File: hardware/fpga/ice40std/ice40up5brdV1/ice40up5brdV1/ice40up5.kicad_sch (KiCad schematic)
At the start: 5 parts, among them U1 ICE40UP5K-SG48ITR

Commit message: pwm / lvds power / filters
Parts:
- C1, C20: footprint Capacitor_SMD:C_0402_1005Metric -> Capacitor_SMD:C_1206_3216Metric
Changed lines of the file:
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@@
       (effects (font (size 1.27 1.27)) (justify left))
     )
-    (property "Footprint" "Capacitor_SMD:C_0402_1005Metric" (id 2) (at 127.9652 53.34 0)
+    (property "Footprint" "Capacitor_SMD:C_1206_3216Metric" (id 2) (at 127.9652 53.34 0)
       (effects (font (size 1.27 1.27)) hide)
     )
@@
       (effects (font (size 1.27 1.27)) (justify left))
     )
-    (property "Footprint" "Capacitor_SMD:C_0402_1005Metric" (id 2) (at 238.4552 58.4075 0)
+    (property "Footprint" "Capacitor_SMD:C_1206_3216Metric" (id 2) (at 238.4552 58.4075 0)
       (effects (font (size 1.27 1.27)) hide)
     )

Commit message: pwm / lvds power / filters
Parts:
- C1, C20: footprint Capacitor_SMD:C_1206_3216Metric -> Capacitor_SMD:C_0603_1608Metric
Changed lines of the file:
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@@
       (effects (font (size 1.27 1.27)) (justify left))
     )
-    (property "Footprint" "Capacitor_SMD:C_1206_3216Metric" (id 2) (at 127.9652 53.34 0)
+    (property "Footprint" "Capacitor_SMD:C_0603_1608Metric" (id 2) (at 127.9652 53.34 0)
       (effects (font (size 1.27 1.27)) hide)
     )
@@
       (effects (font (size 1.27 1.27)) (justify left))
     )
-    (property "Footprint" "Capacitor_SMD:C_1206_3216Metric" (id 2) (at 238.4552 58.4075 0)
+    (property "Footprint" "Capacitor_SMD:C_0603_1608Metric" (id 2) (at 238.4552 58.4075 0)
       (effects (font (size 1.27 1.27)) hide)
     )

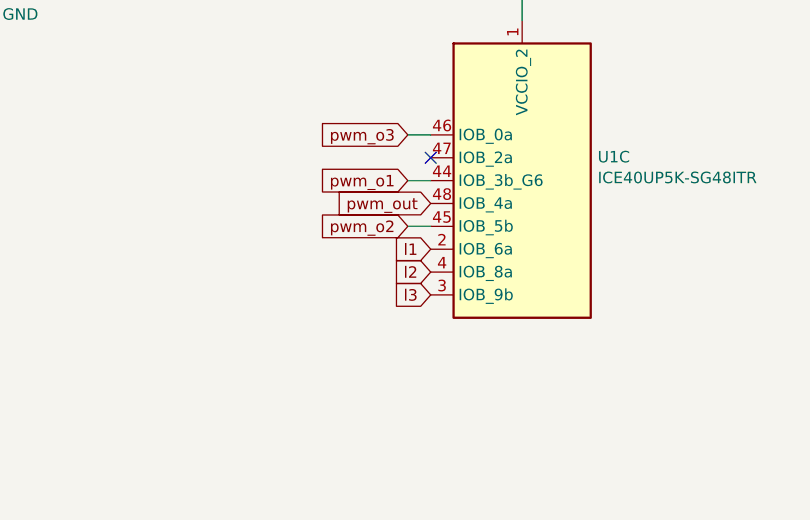
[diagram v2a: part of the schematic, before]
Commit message: pwm / lvds power / filters
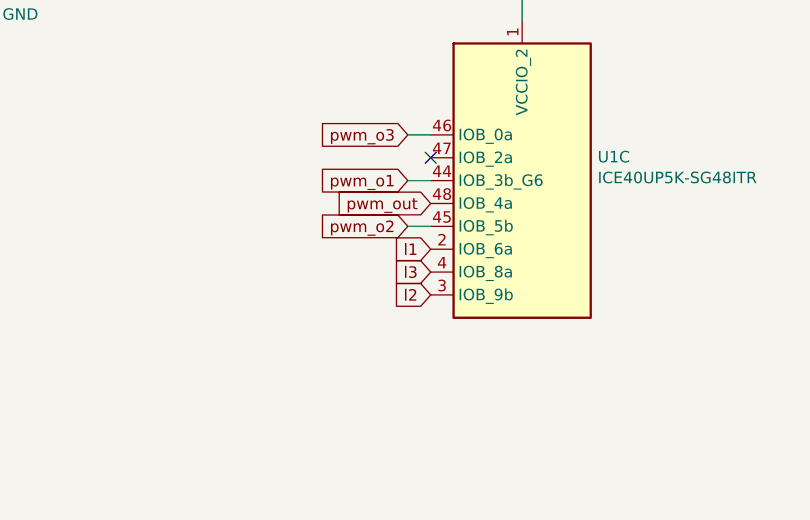
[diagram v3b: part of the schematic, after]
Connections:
- net l2: now also U1.3 (IOB_9b); no longer U1.4 (IOB_8a)
- net l3: now also U1.4 (IOB_8a); no longer U1.3 (IOB_9b)
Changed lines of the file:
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@@
     (stroke (width 0) (type default) (color 0 0 0 0))
   )
-  (global_label "l3" (shape input) (at 179.07 101.6 180) (fields_autoplaced)
+  (global_label "l3" (shape input) (at 179.07 99.06 180) (fields_autoplaced)
     (effects (font (size 1.27 1.27)) (justify right))
-    (property "Intersheet References" "${INTERSHEET_REFS}" (id 0) (at 174.871 101.5206 0)
+    (property "Intersheet References" "${INTERSHEET_REFS}" (id 0) (at 174.871 98.9806 0)
       (effects (font (size 1.27 1.27)) (justify right) hide)
     )
@@
     )
   )
-  (global_label "l2" (shape input) (at 179.07 99.06 180) (fields_autoplaced)
+  (global_label "l2" (shape input) (at 179.07 101.6 180) (fields_autoplaced)
     (effects (font (size 1.27 1.27)) (justify right))
-    (property "Intersheet References" "${INTERSHEET_REFS}" (id 0) (at 174.871 98.9806 0)
+    (property "Intersheet References" "${INTERSHEET_REFS}" (id 0) (at 174.871 101.5206 0)
       (effects (font (size 1.27 1.27)) (justify right) hide)
     )
